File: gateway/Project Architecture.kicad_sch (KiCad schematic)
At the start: 0 parts

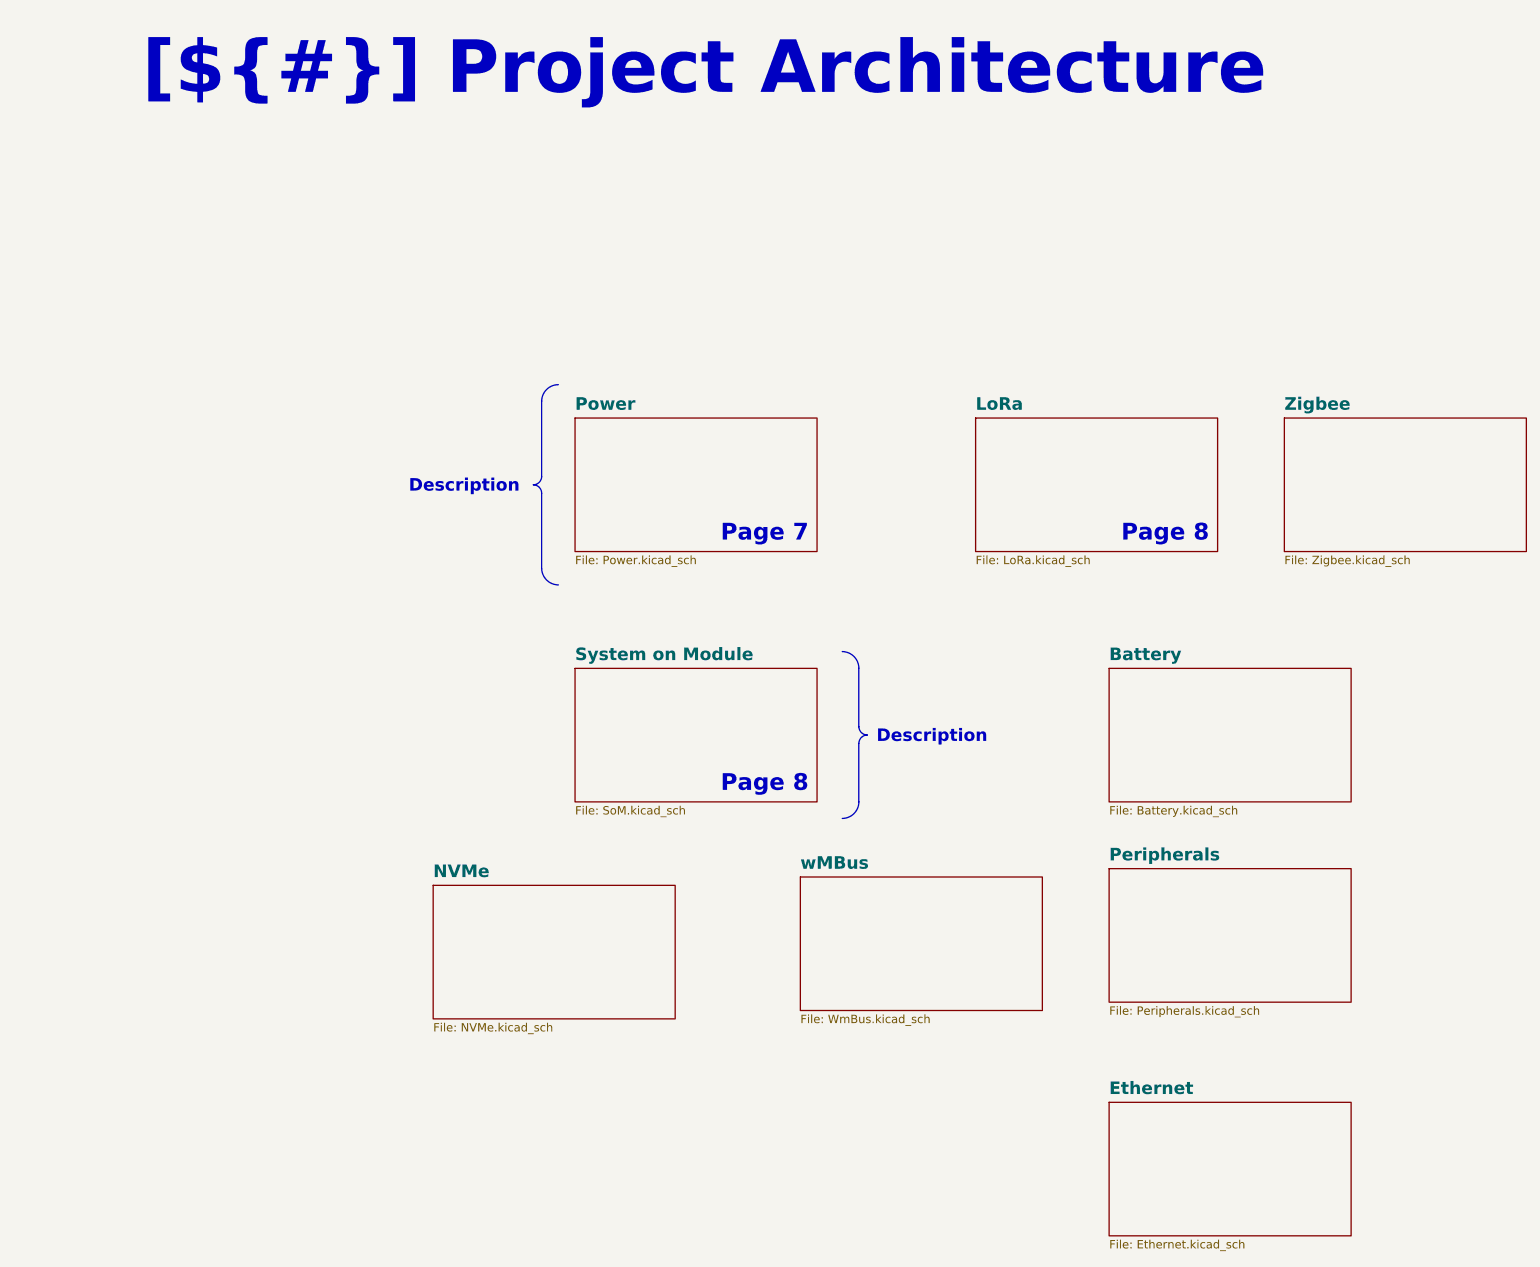
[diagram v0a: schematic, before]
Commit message: Working on PCB
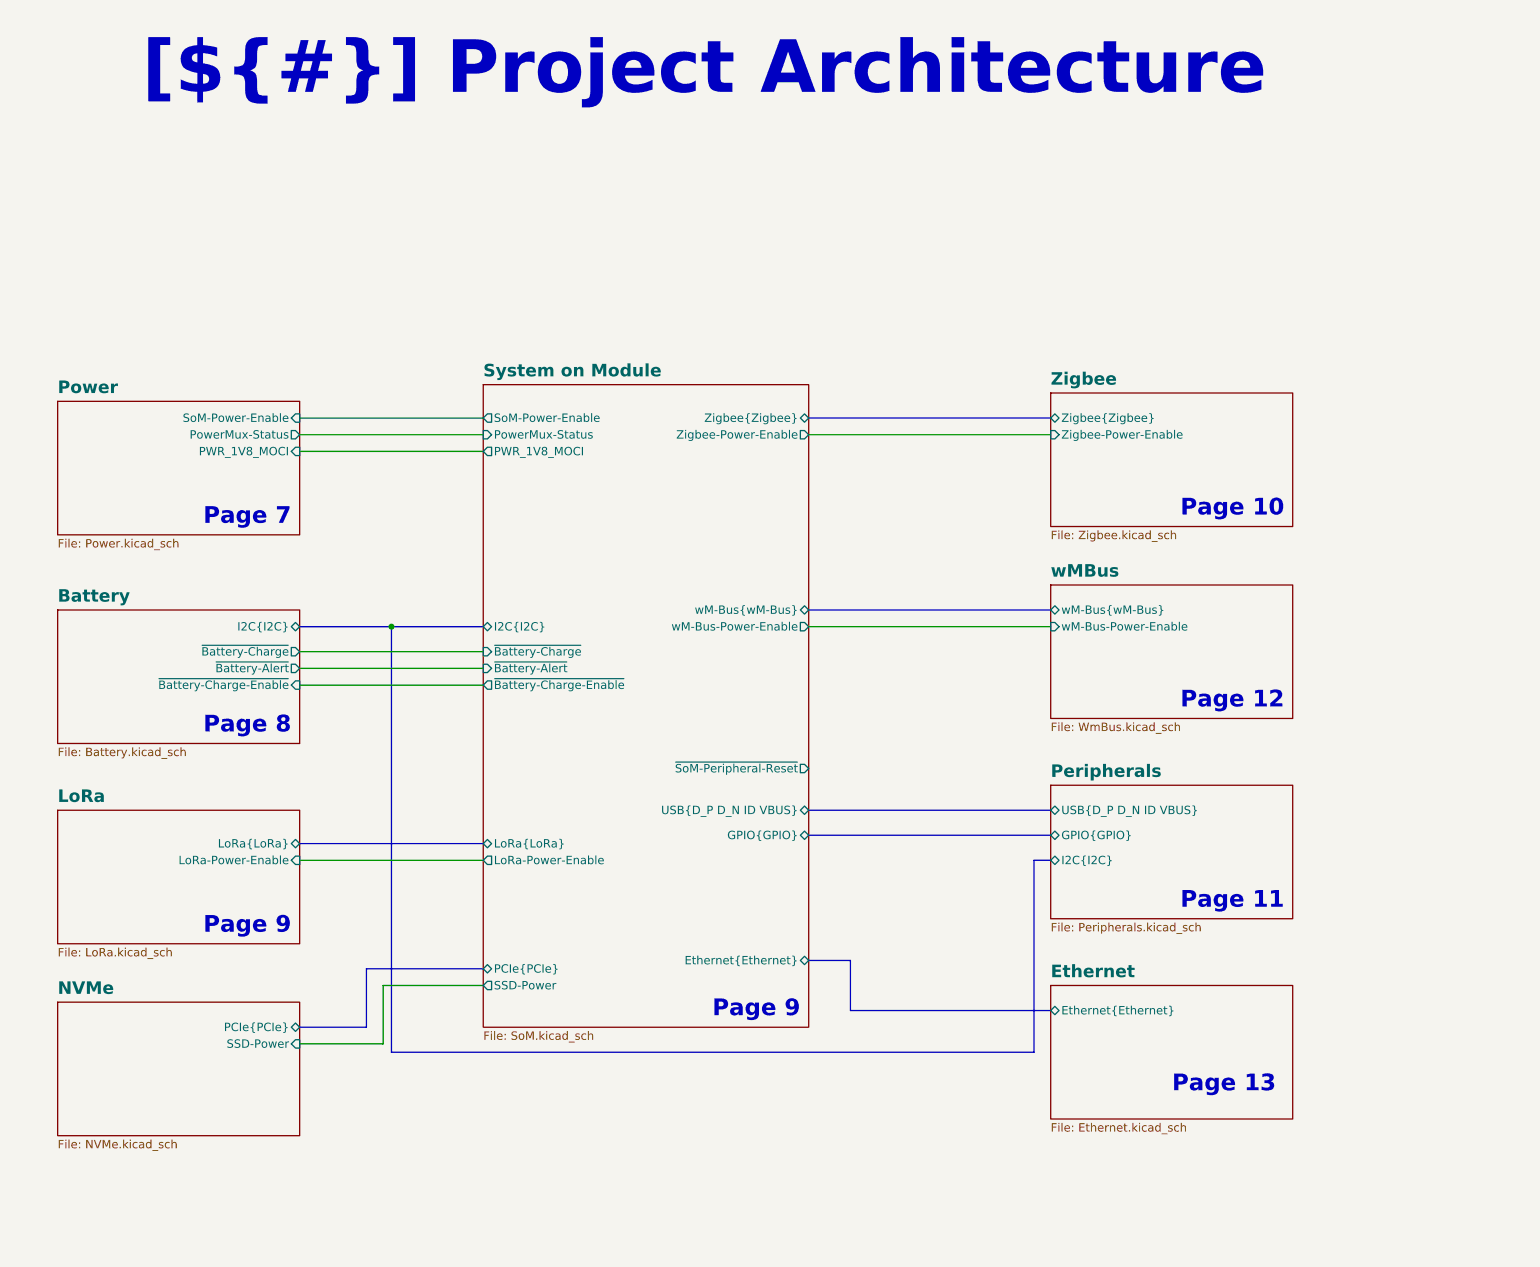
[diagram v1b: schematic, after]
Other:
- sheet Battery ports: added I2C{I2C}, ~{Battery-Alert}, ~{Battery-Charge-Enable}, ~{Battery-Charge}; removed none
- sheet Ethernet ports: added Ethernet{Ethernet}; removed none
- sheet LoRa ports: added LoRa-Power-Enable, LoRa{LoRa}; removed none
- sheet NVMe ports: added PCIe{PCIe}, SSD-Power; removed none
- sheet Peripherals ports: added GPIO{GPIO}, I2C{I2C}, USB{D_P D_N ID VBUS}; removed none
- sheet Power ports: added PWR_1V8_MOCI, PowerMux-Status, SoM-Power-Enable; removed none
- sheet System on Module ports: added Ethernet{Ethernet}, GPIO{GPIO}, I2C{I2C}, LoRa-Power-Enable, LoRa{LoRa}, PCIe{PCIe}, PWR_1V8_MOCI, PowerMux-Status, SSD-Power, SoM-Power-Enable, USB{D_P D_N ID VBUS}, Zigbee-Power-Enable, Zigbee{Zigbee}, wM-Bus-Power-Enable, wM-Bus{wM-Bus}, ~{Battery-Alert}, ~{Battery-Charge-Enable}, ~{Battery-Charge}, ~{SoM-Peripheral-Reset}; removed none
- sheet Zigbee ports: added Zigbee-Power-Enable, Zigbee{Zigbee}; removed none
- sheet wMBus ports: added wM-Bus-Power-Enable, wM-Bus{wM-Bus}; removed none
- note added: "Page 10"
- note added: "Page 11"
- note added: "Page 12"
- note added: "Page 13"
- note added: "Page 9"
